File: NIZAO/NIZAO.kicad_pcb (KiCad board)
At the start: 4 copper layers, 107 x 87.7 mm, 180 parts, among them J1 Screw_Terminal_01x09, J2 Screw_Terminal_01x09, J3 Screw_Terminal_01x09, J4 Screw_Terminal_01x09, J5 PZ254R-12-14P, K1 G5V-1, K2 G5V-1, Q1 NCE60P04R, Q2 ZXMS6004FFQTA, Q3 ZXMS6004FFQTA, Q4 ZXMS6004FFQTA, Q5 ZXMS6004FFQTA, SW1 TS-1088-AR02016, U1 ADS1115IDGS, U10 AT3H4B-CUH-S, U11 MAX31856MUD+, U12 BL0942, U13 B0303S-1WR3_C7465185, U14 ISO7021DR, U15 GP8211S-TC50-EW, U16 GP8302-TC50-EW, U17 BTS723GWXUMA1, U18 LK1802, U2 ESP32-S3-WROOM-1, U3 RS485-PROTECT, U4 AP63203WU, U5 AT3H4B-CUH-S, U6 AT3H4B-CUH-S, U7 AT3H4B-CUH-S, U8 AT3H4B-CUH-S, U9 AT3H4B-CUH-S

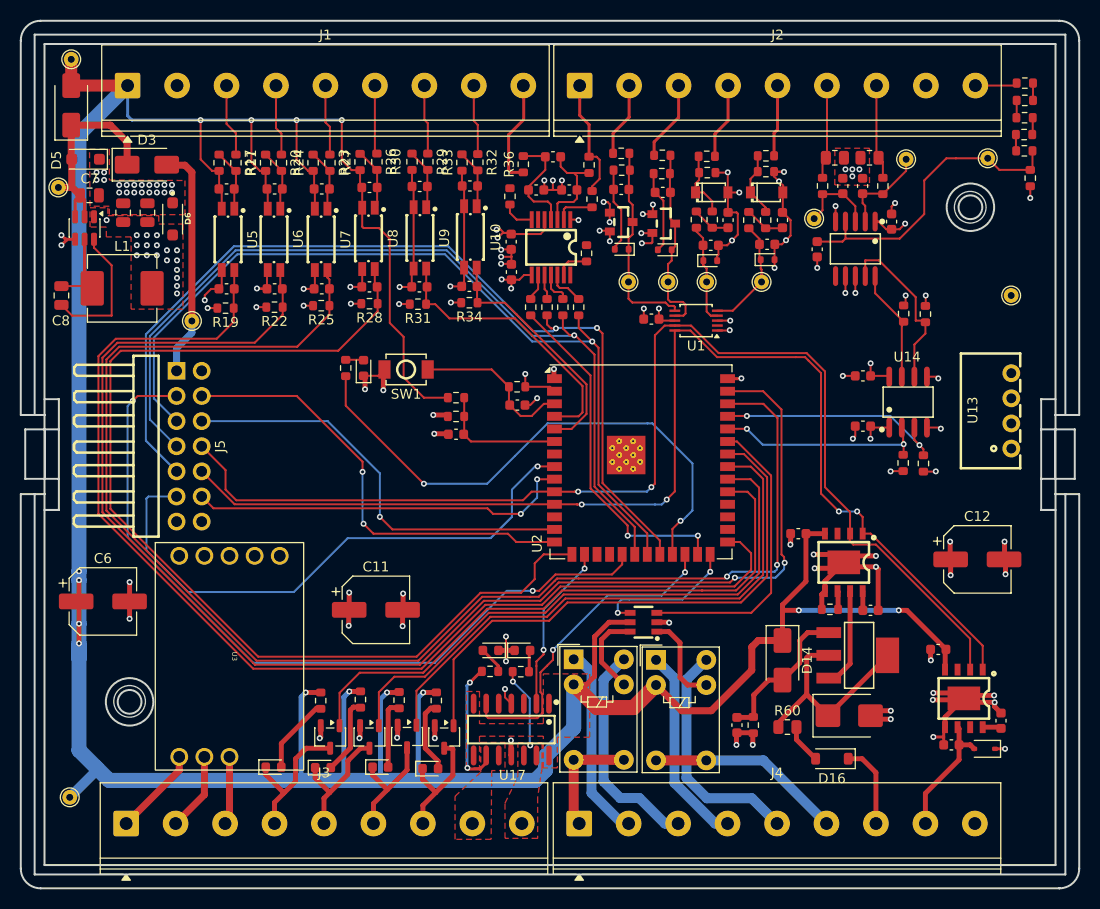
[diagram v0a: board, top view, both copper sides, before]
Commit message: actualizacion
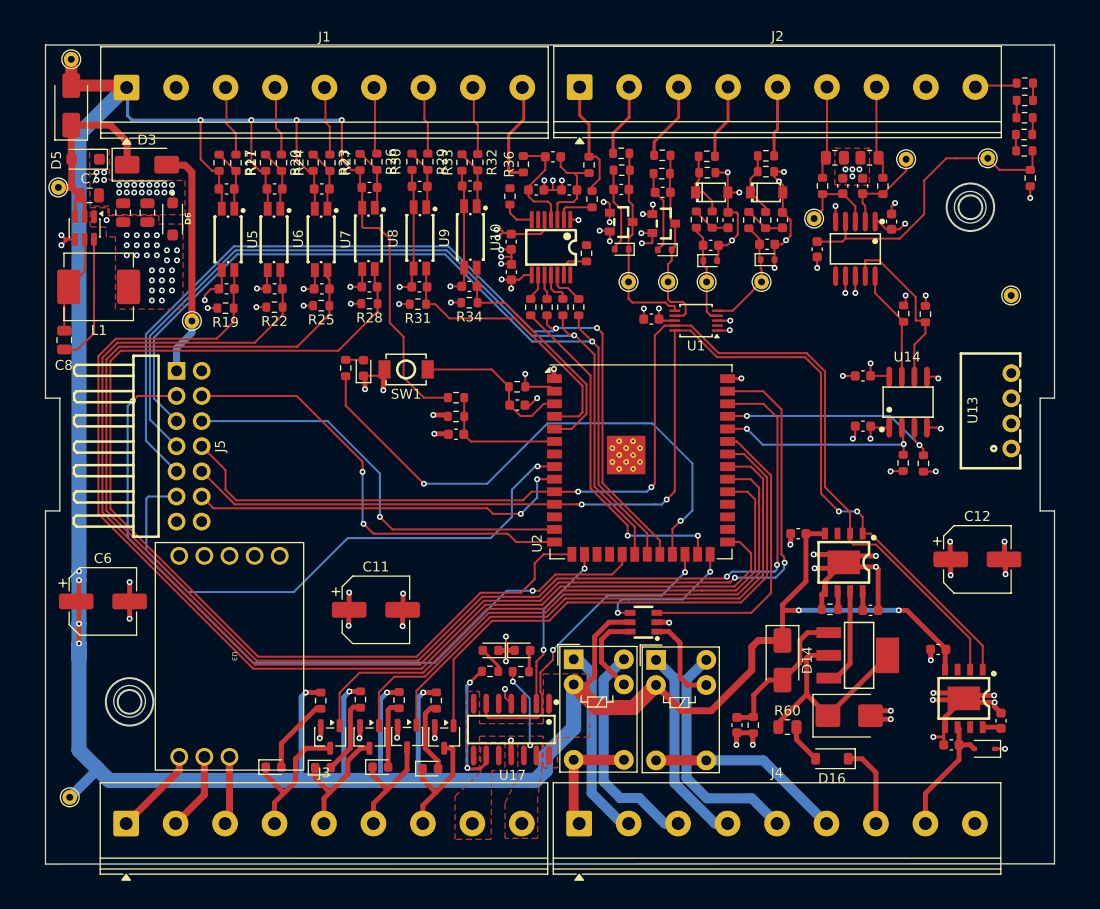
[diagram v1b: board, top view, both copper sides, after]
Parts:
- moved C8 4.52 mm to (102.4, 85.3)
- moved L1 2.38 mm to (105.9, 79.9)
- moved J1 0.22 mm to (108.7, 59.8)
- moved J2 0.15 mm to (154.5, 59.7)
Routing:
- net /PawerSupply/sw: track 8.49 -> 10.1 mm
- net Net-(U4-BST): track 14.0 -> 13.2 mm
- net +3.3V: vias 42 -> 52
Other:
- board size 107 x 87.7 mm -> 102 x 82.8 mm
